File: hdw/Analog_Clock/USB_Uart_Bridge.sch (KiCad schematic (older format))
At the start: 39 parts, among them J1301 USB_B_Mini, U1301 TLV6700, U1302 FT234XD, U1303 74LVC1G17, U1304 TXB0102DCU, U1305 TPD3S014DBVR

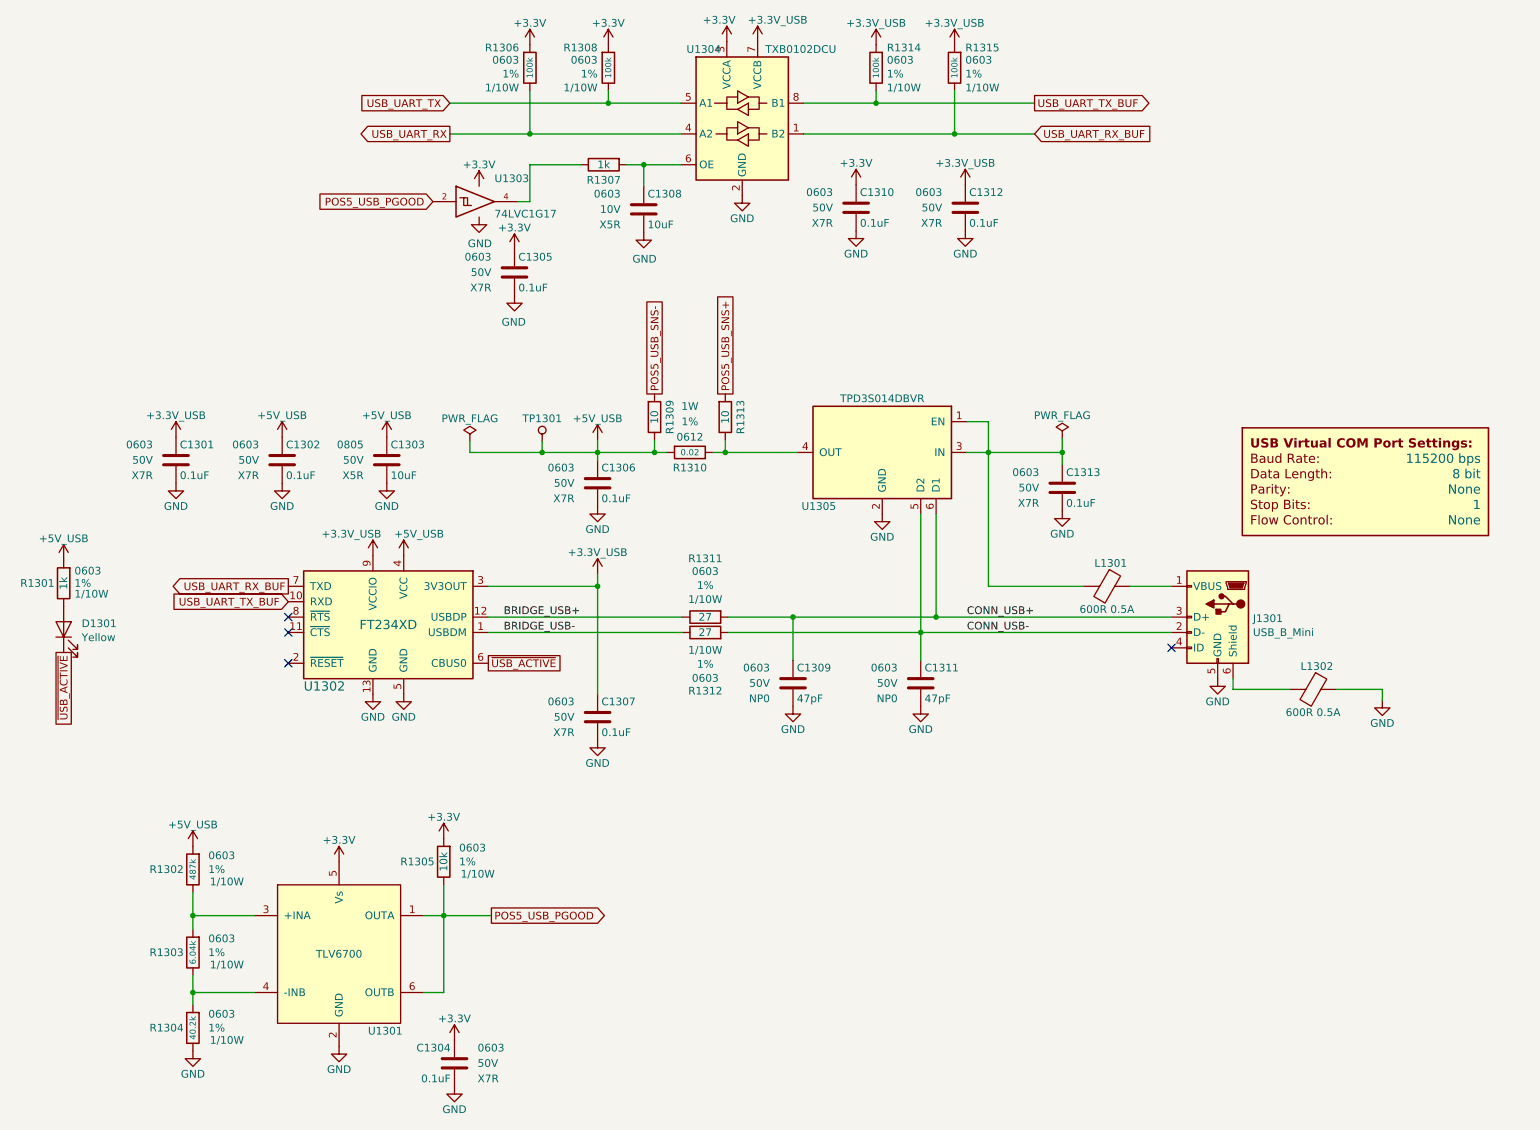
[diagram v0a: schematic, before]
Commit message: More PCB arrangement
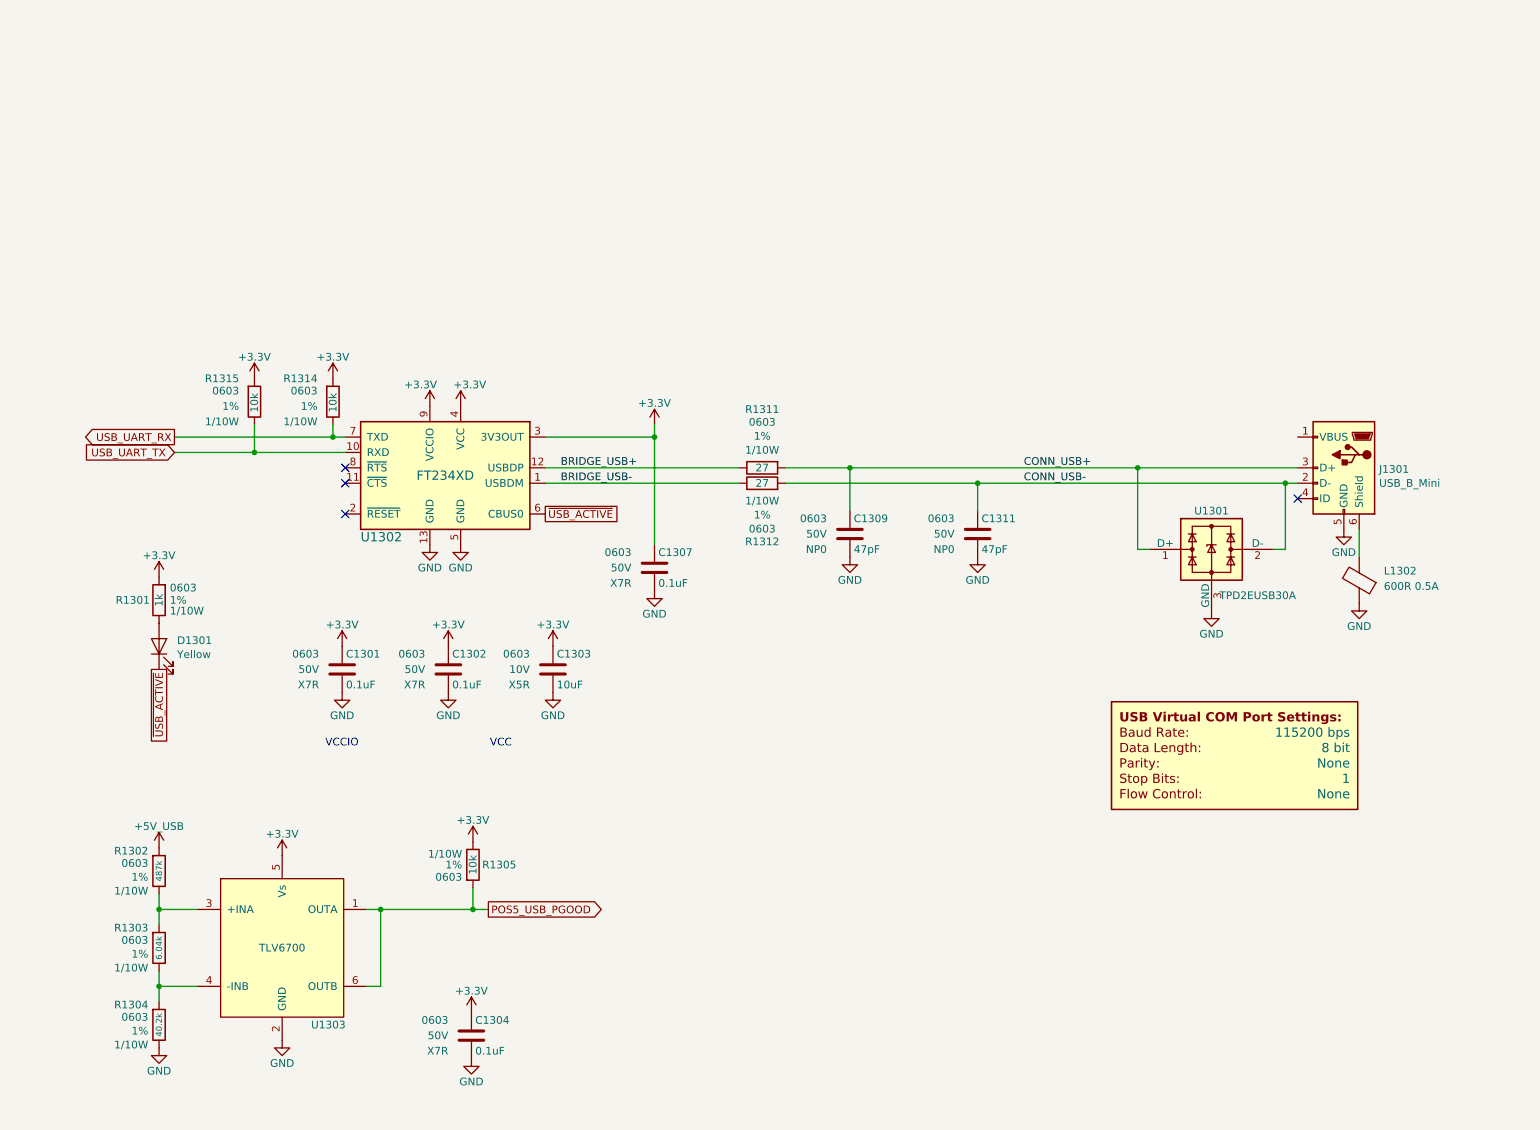
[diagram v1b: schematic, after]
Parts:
- removed C1305, C1306, C1310, C1312, C1313: 0.1uF, Capacitors_SMD:C_0603, symbol Custom_Library:C_Custom
- removed C1308: 10uF, Capacitors_SMD:C_0603, symbol Custom_Library:C_Custom
- removed L1301: 600R 0.5A, Inductors_SMD:L_0603, symbol Device:Ferrite_Bead
- removed R1306, R1308: 100k, Resistors_SMD:R_0603, symbol Custom_Library:R_Custom
- removed R1307: 1k, Resistors_SMD:R_0603, symbol Custom_Library:R_Custom
- removed R1309, R1313: 10, Resistors_SMD:R_0603, symbol Custom_Library:R_Custom
- removed R1310: 0.02, Resistors_SMD:R_0612, symbol Custom_Library:R_Custom
- removed TP1301: TP, Custom Footprints Library:Test_Point, symbol Custom_Library:TP
- removed U1301: TLV6700, Package_TO_SOT_SMD:SOT-23-6, symbol Custom_Library:TLV6700
- removed U1303: 74LVC1G17, TO_SOT_Packages_SMD:SOT-353_SC-70-5, symbol Custom_Library:74LVC1G17_Power
- removed U1304: TXB0102DCU, Package_SO:VSSOP-8_2.4x2.1mm_P0.5mm, symbol Logic_LevelTranslator:TXB0102DCU
- removed U1305: TPD3S014DBVR, TO_SOT_Packages_SMD:SOT-23-6, symbol Custom_Library:TPD3S014DBVR
- added U1301: TPD2EUSB30A, Package_TO_SOT_SMD:Texas_DRT-3, symbol Power_Protection:TPD2EUSB30A
- added U1303: TLV6700, Package_TO_SOT_SMD:SOT-23-6, symbol Custom_Library:TLV6700
- C1303: footprint Capacitors_SMD:C_0805 -> Capacitors_SMD:C_0603; Digi-Key PN 490-18664-1-ND -> 490-10474-1-ND; Voltage 50V -> 10V; display_footprint 0805 -> 0603
- R1302: Digi-Key PN 311-487KHRCT-ND -> (none)
- R1303: Digi-Key PN RMCF0603FT6K04CT-ND -> (none)
- R1304: Digi-Key PN RMCF0603FT40K2CT-ND -> (none)
- R1314, R1315: value 100k -> 10k; Digi-Key PN RMCF0603FT100KCT-ND -> YAG2321CT-ND
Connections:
- net +3.3V_USB is gone; now on net +3V3: C1301.1, C1307.1, R1314.1, R1315.1, U1302.3 (3V3OUT), U1302.9 (VCCIO)
- net +3V3: now also C1302.1, C1303.1, R1301.1, R1305.2, U1302.4 (VCC), U1303.5 (Vs); no longer R1305.1
- net +5V_USB: no longer C1302.1, C1303.1, R1301.1, U1302.4 (VCC)
- net CONN_USB+: now also U1301.1 (D+)
- net CONN_USB-: now also U1301.2 (D-)
- net GND: now also U1301.3 (GND), U1303.2 (GND)
- net POS5_USB_PGOOD: now also R1305.1, U1303.1 (OUTA), U1303.6 (OUTB); no longer R1305.2
- net USB_UART_RX: now also R1314.2, U1302.7 (TXD)
- net USB_UART_TX: now also R1315.2, U1302.10 (RXD)
- net at R1302.2, R1303.1: now also U1303.3 (+INA)
- net at R1303.2, R1304.1: now also U1303.4 (-INB)
- removed net USB_UART_RX_BUF: R1315.2, U1302.7 (TXD)
- removed net USB_UART_TX_BUF: R1314.2, U1302.10 (RXD)
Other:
- note added: "VCC"
- note added: "VCCIO"
- moved on the sheet: C1301, C1302, C1307, C1309, C1311, D1301, J1301, L1302, R1301, R1311, R1312, U1302
